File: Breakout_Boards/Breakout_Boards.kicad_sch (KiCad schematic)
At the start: 3 parts, among them J1 2xRJ_45, J2 Conn_01x06_Pin, J3 Conn_01x06_Pin

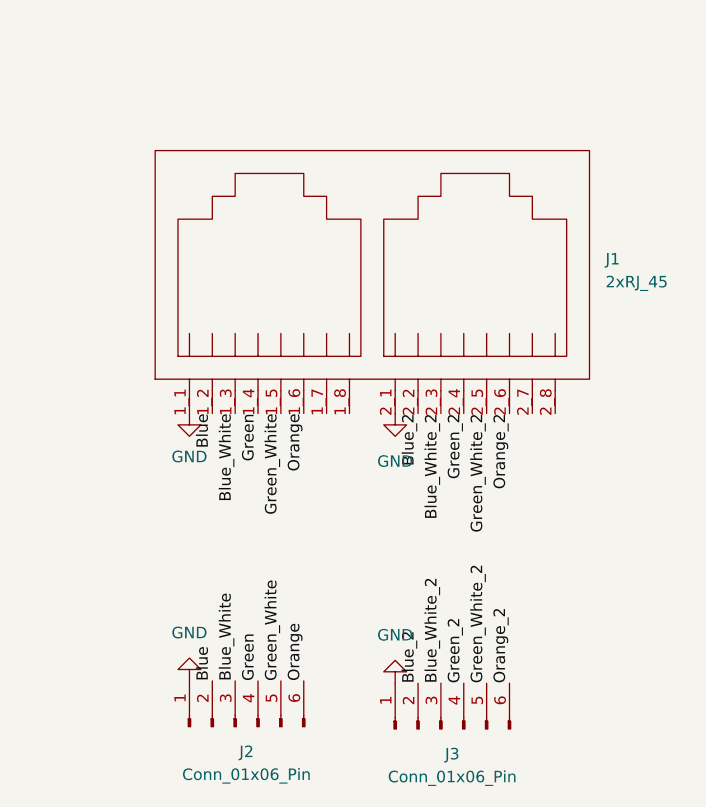
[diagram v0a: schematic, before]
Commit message: Active Electrode
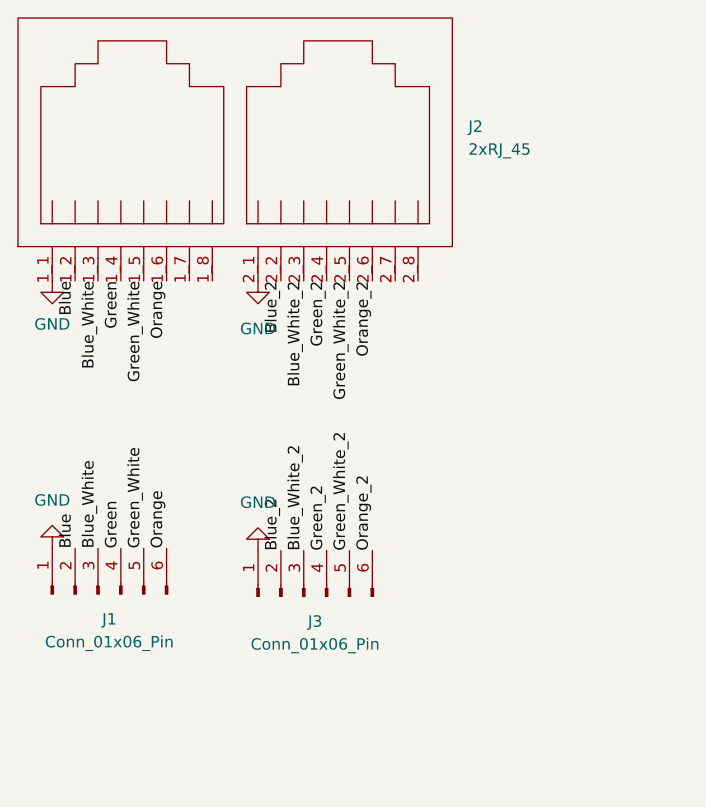
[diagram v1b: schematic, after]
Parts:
- removed J1: 2xRJ_45, TE_2xRJ45:TE_2xRJ45, symbol Duel_Ethernet_Port:Duel_Ethernet_Port
- removed J2: Conn_01x06_Pin, Connector_PinSocket_2.54mm:PinSocket_1x06_P2.54mm_Vertical, symbol Connector:Conn_01x06_Pin
- added J1: Conn_01x06_Pin, Connector_PinSocket_2.54mm:PinSocket_1x06_P2.54mm_Vertical, symbol Connector:Conn_01x06_Pin
- added J2: 2xRJ_45, TE_2xRJ45:TE_2xRJ45, symbol Duel_Ethernet_Port:Duel_Ethernet_Port
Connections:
- net Blue: now also J1.2 (Pin_2), J2.1_2
- net Blue_2: now also J2.2_2
- net Blue_White: now also J1.3 (Pin_3), J2.1_3
- net Blue_White_2: now also J2.2_3
- net GND: now also J1.1 (Pin_1), J2.1_1, J2.2_1
- net Green: now also J1.4 (Pin_4), J2.1_4
- net Green_2: now also J2.2_4
- net Green_White: now also J1.5 (Pin_5), J2.1_5
- net Green_White_2: now also J2.2_5
- net Orange: now also J1.6 (Pin_6), J2.1_6
- net Orange_2: now also J2.2_6
